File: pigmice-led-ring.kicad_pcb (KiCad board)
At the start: 2 copper layers, 46 x 51 mm, 46 parts, among them J1 Conn_01x02_Female, J2 Conn_01x03_Female, U1 LMR62014XMF

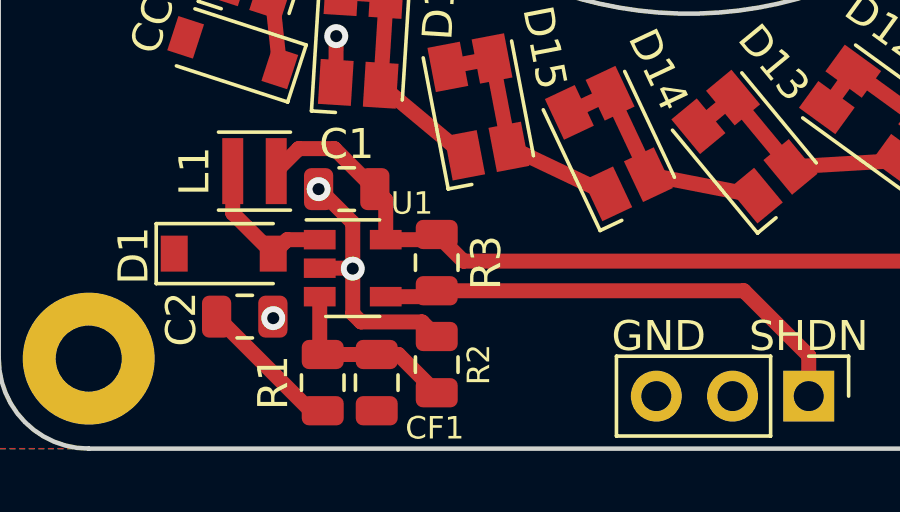
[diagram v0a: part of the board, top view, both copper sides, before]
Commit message: Move labels a bit
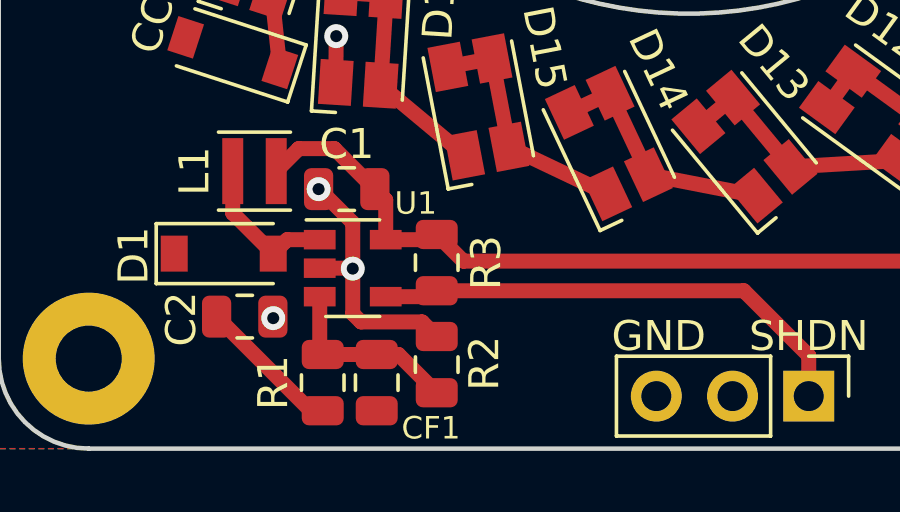
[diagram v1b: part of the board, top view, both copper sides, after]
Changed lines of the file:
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@@
     (tags SOT-23-5)
     (attr smd)
-    (fp_text reference U1 (at 1.972 -2.162839) (layer F.SilkS)
+    (fp_text reference U1 (at 2.099 -2.162839) (layer F.SilkS)
       (effects (font (size 0.75 0.75) (thickness 0.15)))
     )
@@
     (tags resistor)
     (attr smd)
-    (fp_text reference R2 (at 0 1.4 270) (layer F.SilkS)
-      (effects (font (size 0.75 0.75) (thickness 0.15)))
+    (fp_text reference R2 (at 0.044 1.585 270) (layer F.SilkS)
+      (effects (font (size 1 1) (thickness 0.15)))
     )
     (fp_text value 13.3k (at 0 1.65 90) (layer F.Fab)
@@
     (tags capacitor)
     (attr smd)
-    (fp_text reference CF1 (at 1.515 -1.934) (layer F.SilkS)
+    (fp_text reference CF1 (at 1.515 -1.807) (layer F.SilkS)
       (effects (font (size 0.75 0.75) (thickness 0.15)))
     )
